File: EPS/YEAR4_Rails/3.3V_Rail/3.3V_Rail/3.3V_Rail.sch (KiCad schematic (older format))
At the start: 20 parts, among them J1 Conn_01x02, J2 Conn_01x02, J3 Conn_01x02, J4 Conn_01x02, J5 Conn_01x02, J6 Conn_01x02, J7 Conn_01x02_Female

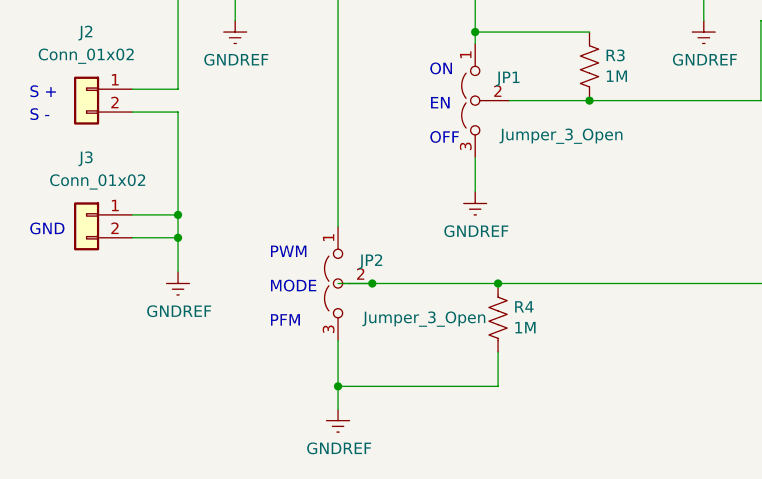
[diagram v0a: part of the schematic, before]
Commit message: Update 3.3V_Rail.sch
Update v.0.1
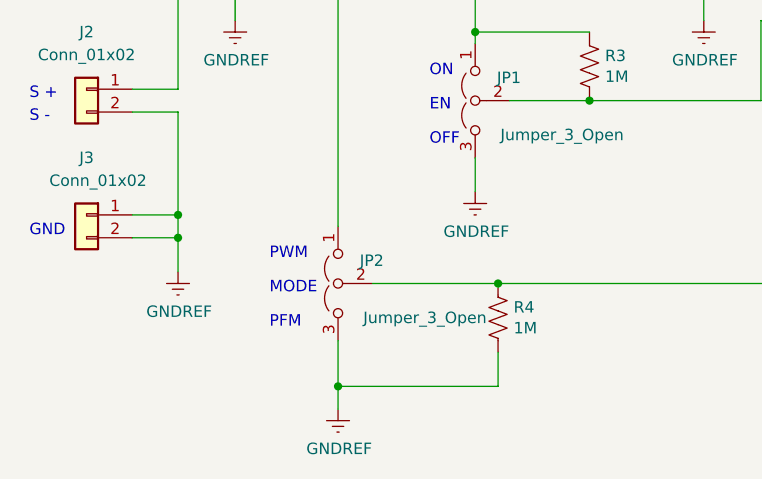
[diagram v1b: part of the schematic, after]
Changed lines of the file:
@@
 	2500 2400 3100 2400
-Wire Wire Line
-	2500 3850 2650 3850
-Connection ~ 2650 3850
 Wire Wire Line
 	2650 3850 3200 3850
